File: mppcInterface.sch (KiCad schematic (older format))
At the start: 12 parts, among them J9 Raspberry_Pi_2_3, U1 DAC60508ZRTE, U14 ICE40-LP384-SG32, U2 74HC14, U3 74HC14, U4 INA285

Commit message: Max1932 routed, fpga signal in router. Going to removed Voltage div here
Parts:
- removed D1: S13360-2050VE, s13360-2050ve:S13360-2050VE, symbol s13360-2050ve:S13360-2050VE
- removed R1: 4K99, Resistor_SMD:R_0402_1005Metric, symbol Device:R_US
- removed U2, U3: 74HC14, Package_SO:SOIC-14_3.9x8.7mm_P1.27mm, symbol 74xx:74HC14
- removed U4: INA285, ina28x:TI-DGK-VSSOP-8, symbol ina28x:INA285
- added D1: D, Diode_SMD:D_0402_1005Metric, symbol Device:D
- added TP10: CH5, TestPoint:TestPoint_Bridge_Pitch2.0mm_Drill0.7mm, symbol Connector:TestPoint
- added TP11: CH6, TestPoint:TestPoint_Bridge_Pitch2.0mm_Drill0.7mm, symbol Connector:TestPoint
- added TP12: CH7, TestPoint:TestPoint_Bridge_Pitch2.0mm_Drill0.7mm, symbol Connector:TestPoint
- added TP5: CH0, TestPoint:TestPoint_Bridge_Pitch2.0mm_Drill0.7mm, symbol Connector:TestPoint
- added TP6: CH1, TestPoint:TestPoint_Bridge_Pitch2.0mm_Drill0.7mm, symbol Connector:TestPoint
- added TP7: CH2, TestPoint:TestPoint_Bridge_Pitch2.0mm_Drill0.7mm, symbol Connector:TestPoint
- added TP8: CH3, TestPoint:TestPoint_Bridge_Pitch2.0mm_Drill0.7mm, symbol Connector:TestPoint
- added TP9: CH4, TestPoint:TestPoint_Bridge_Pitch2.0mm_Drill0.7mm, symbol Connector:TestPoint
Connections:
- net labels removed: CH0-A, CH1-A, CH2-A, CH3-A, CH4-A, CH5-A, CH6-A, CH7-A, VBUS
- wire segments 118 -> 123
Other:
- moved on the sheet: U14

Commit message: -5v supply, fpga routed
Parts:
- added C22, C24: 10u, Capacitor_SMD:C_0402_1005Metric, symbol Device:C
- added C23: 1u, Capacitor_SMD:C_0402_1005Metric, symbol Device:C
- added TP2: GND, TestPoint:TestPoint_Bridge_Pitch2.0mm_Drill0.7mm, symbol Connector:TestPoint
- added U2: MIC5504-1.2YM5, Package_TO_SOT_SMD:SOT-23-5, symbol Regulator_Linear:MIC5504-1.2YM5
- added U3: LM2776, Package_TO_SOT_SMD:SOT-23-6, symbol Regulator_SwitchedCapacitor:LM2776
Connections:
- net labels added: -5V
- wire segments 123 -> 147
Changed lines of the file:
@@
 Wire Wire Line
 	6250 4650 6350 4650
+$Comp
+L Regulator_Linear:MIC5504-1.2YM5 U2
+U 1 1 5C3A61F2
+P 1850 6000
+F 0 "U2" H 1850 6367 50  0000 C CNN
+F 1 "MIC5504-1.2YM5" H 1850 6276 50  0000 C CNN
+F 2 "Package_TO_SOT_SMD:SOT-23-5" H 1850 5600 50  0001 C CNN
+F 3 "http://ww1.microchip.com/downloads/en/DeviceDoc/MIC550X.pdf" H 1600 6250 50  0001 C CNN
+	1    1850 6000
+	1    0    0    -1
+$EndComp
+$Comp
+L power:+3V3 #PWR0105
+U 1 1 5C3A62A7
+P 1350 5900
+F 0 "#PWR0105" H 1350 5750 50  0001 C CNN
+F 1 "+3V3" H 1365 6073 50  0000 C CNN
+F 2 "" H 1350 5900 50  0001 C CNN
+F 3 "" H 1350 5900 50  0001 C CNN
+	1    1350 5900
+	1    0    0    -1
+$EndComp
+$Comp
+L power:GND #PWR0106
+U 1 1 5C3A62D4
+P 1850 6350
+F 0 "#PWR0106" H 1850 6100 50  0001 C CNN
+F 1 "GND" H 1855 6177 50  0000 C CNN
+F 2 "" H 1850 6350 50  0001 C CNN
+F 3 "" H 1850 6350 50  0001 C CNN
+	1    1850 6350
+	1    0    0    -1
+$EndComp
+$Comp
+L power:+1V2 #PWR0107
+U 1 1 5C3A6301
+P 2300 5850
+F 0 "#PWR0107" H 2300 5700 50  0001 C CNN
+F 1 "+1V2" H 2315 6023 50  0000 C CNN
+F 2 "" H 2300 5850 50  0001 C CNN
+F 3 "" H 2300 5850 50  0001 C CNN
+	1    2300 5850
+	1    0    0    -1
+$EndComp
+Wire Wire Line
+	1450 6100 1400 6100
+Wire Wire Line
+	1400 6100 1400 5900
+Wire Wire Line
+	1400 5900 1450 5900
+Wire Wire Line
+	2300 5850 2300 5900
+Wire Wire Line
+	2300 5900 2250 5900
+Wire Wire Line
+	1850 6350 1850 6300
+Wire Wire Line
+	1350 5900 1400 5900
+Connection ~ 1400 5900
+$Comp
+L Connector:TestPoint TP?
+U 1 1 5C3D0D7D
+P 10400 5200
+AR Path="/5C210B26/5C3D0D7D" Ref="TP?"  Part="1"
+AR Path="/5C3D0D7D" Ref="TP2"  Part="1"
+F 0 "TP2" H 10458 5320 50  0000 L CNN
+F 1 "GND" H 10458 5229 50  0000 L CNN
+F 2 "TestPoint:TestPoint_Bridge_Pitch2.0mm_Drill0.7mm" H 10600 5200 50  0001 C CNN
+F 3 "~" H 10600 5200 50  0001 C CNN
+	1    10400 5200
+	1    0    0    -1
+$EndComp
+$Comp
+L power:GND #PWR0108
+U 1 1 5C3D0E0F
+P 10400 5250
+F 0 "#PWR0108" H 10400 5000 50  0001 C CNN
+F 1 "GND" H 10405 5077 50  0000 C CNN
+F 2 "" H 10400 5250 50  0001 C CNN
+F 3 "" H 10400 5250 50  0001 C CNN
+	1    10400 5250
+	1    0    0    -1
+$EndComp
+Wire Wire Line
+	10400 5200 10400 5250
+$Comp
+L Regulator_SwitchedCapacitor:LM2776 U3
+U 1 1 5C3D6E4F
+P 2200 4500
+F 0 "U3" H 2350 4300 50  0000 L CNN
+F 1 "LM2776" H 2100 4450 50  0000 L CNN
+F 2 "Package_TO_SOT_SMD:SOT-23-6" H 2250 4150 50  0001 L CNN
+F 3 "http://www.ti.com/lit/ds/symlink/lm2776.pdf" H 350 5750 50  0001 C CNN
+	1    2200 4500
+	1    0    0    -1
+$EndComp
+$Comp
+L power:+5V #PWR0109
+U 1 1 5C3D75DC
+P 2200 4100
+F 0 "#PWR0109" H 2200 3950 50  0001 C CNN
+F 1 "+5V" H 2215 4273 50  0000 C CNN
+F 2 "" H 2200 4100 50  0001 C CNN
+F 3 "" H 2200 4100 50  0001 C CNN
+	1    2200 4100
+	1    0    0    -1
+$EndComp
+$Comp
+L power:GND #PWR0110
+U 1 1 5C3D760D
+P 2200 4950
+F 0 "#PWR0110" H 2200 4700 50  0001 C CNN
+F 1 "GND" H 2205 4777 50  0000 C CNN
+F 2 "" H 2200 4950 50  0001 C CNN
+F 3 "" H 2200 4950 50  0001 C CNN
+	1    2200 4950
+	1    0    0    -1
+$EndComp
+$Comp
+L power:-5V #PWR0111
+U 1 1 5C3D765C
+P 2650 4350
+F 0 "#PWR0111" H 2650 4450 50  0001 C CNN
+F 1 "-5V" H 2665 4523 50  0000 C CNN
+F 2 "" H 2650 4350 50  0001 C CNN
+F 3 "" H 2650 4350 50  0001 C CNN
+	1    2650 4350
+	1    0    0    -1
+$EndComp
+Wire Wire Line
+	1800 4400 1750 4400
+Wire Wire Line
+	1750 4400 1750 4150
+Wire Wire Line
+	1750 4150 2200 4150
+Wire Wire Line
+	2200 4150 2200 4200
+Wire Wire Line
+	2200 4150 2200 4100
+Connection ~ 2200 4150
+Wire Wire Line
+	2600 4400 2650 4400
+Wire Wire Line
+	2650 4400 2650 4350
+Wire Wire Line
+	2200 4900 2200 4950
+$Comp
+L power:GND #PWR0112
+U 1 1 5C3FB554
+P 2650 4950
+F 0 "#PWR0112" H 2650 4700 50  0001 C CNN
+F 1 "GND" H 2655 4777 50  0000 C CNN
+F 2 "" H 2650 4950 50  0001 C CNN
+F 3 "" H 2650 4950 50  0001 C CNN
+	1    2650 4950
+	1    0    0    -1
+$EndComp
+$Comp
+L Device:C C23
+U 1 1 5C3FC376
+P 1650 4650
+AR Path="/5C3FC376" Ref="C23"  Part="1"
+AR Path="/5C210B26/5C3FC376" Ref="C?"  Part="1"
+F 0 "C23" H 1450 4700 50  0000 L CNN
+F 1 "1u" H 1450 4600 50  0000 L CNN
+F 2 "Capacitor_SMD:C_0402_1005Metric" H 1688 4500 50  0001 C CNN
+F 3 "~" H 1650 4650 50  0001 C CNN
+	1    1650 4650
+	1    0    0    -1
+$EndComp
+$Comp
+L Device:C C24
+U 1 1 5C4024E4
+P 2650 4600
+AR Path="/5C4024E4" Ref="C24"  Part="1"
+AR Path="/5C210B26/5C4024E4" Ref="C?"  Part="1"
+F 0 "C24" H 2750 4650 50  0000 L CNN
+F 1 "10u" H 2750 4550 50  0000 L CNN
+F 2 "Capacitor_SMD:C_0402_1005Metric" H 2688 4450 50  0001 C CNN
+F 3 "~" H 2650 4600 50  0001 C CNN
+	1    2650 4600
+	1    0    0    -1
+$EndComp
+$Comp
+L Device:C C22
+U 1 1 5C402572
+P 1300 4650
+AR Path="/5C402572" Ref="C22"  Part="1"
+AR Path="/5C210B26/5C402572" Ref="C?"  Part="1"
+F 0 "C22" H 1100 4700 50  0000 L CNN
+F 1 "10u" H 1050 4600 50  0000 L CNN
+F 2 "Capacitor_SMD:C_0402_1005Metric" H 1338 4500 50  0001 C CNN
+F 3 "~" H 1300 4650 50  0001 C CNN
+	1    1300 4650
+	1    0    0    -1
+$EndComp
+Wire Wire Line
+	1650 4500 1800 4500
+Wire Wire Line
+	1800 4700 1800 4800
+Wire Wire Line
+	1800 4800 1650 4800
+Wire Wire Line
+	2650 4950 2650 4750
+Wire Wire Line
+	2650 4450 2650 4400
+Connection ~ 2650 4400
+$Comp
+L power:GND #PWR0113
+U 1 1 5C41C31D
+P 1300 4900
+F 0 "#PWR0113" H 1300 4650 50  0001 C CNN
+F 1 "GND" H 1305 4727 50  0000 C CNN
+F 2 "" H 1300 4900 50  0001 C CNN
+F 3 "" H 1300 4900 50  0001 C CNN
+	1    1300 4900
+	1    0    0    -1
+$EndComp
+Wire Wire Line
+	1750 4400 1300 4400
+Wire Wire Line
+	1300 4400 1300 4500
+Connection ~ 1750 4400
+Wire Wire Line
+	1300 4800 1300 4900
 Wire Bus Line
 	8750 800  8750 4600

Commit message: Wired up board
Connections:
- net labels added: CLK, GPIO17, GPIO18, GPIO23, GPIO27, RXD, SDA, SDL, TXD
- wire segments 147 -> 169
- no-connect marks 3 -> 8
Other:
- moved on the sheet: TP2

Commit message: Changed inverter IC, added some decoupling
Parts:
- removed C22, C24: 10u, Capacitor_SMD:C_0402_1005Metric, symbol Device:C
- removed C23: 1u, Capacitor_SMD:C_0402_1005Metric, symbol Device:C
- removed D1: D, Diode_SMD:D_0402_1005Metric, symbol Device:D
- removed U3: LM2776, Package_TO_SOT_SMD:SOT-23-6, symbol Regulator_SwitchedCapacitor:LM2776
- added C22, C24: 10u, Capacitor_SMD:C_0402_1005Metric, symbol mppcInterface-rescue:C-Device
- added C23: 1u, Capacitor_SMD:C_0402_1005Metric, symbol mppcInterface-rescue:C-Device
- added C65: 3u3, Capacitor_SMD:C_0402_1005Metric, symbol mppcInterface-rescue:C-Device
- added R1: 1M13, Resistor_SMD:R_0402_1005Metric, symbol Device:R_US
- added R11: 499k, Resistor_SMD:R_0402_1005Metric, symbol Device:R_US
- added U3: LM27761, Package_SON:WSON-8-1EP_2x2mm_P0.5mm_EP0.9x1.6mm, symbol Regulator_SwitchedCapacitor:LM27761
- H1, H2, H3, H4: symbol Mechanical:MountingHole -> mppcInterface-rescue:MountingHole-Mechanical
- J9: symbol Connector:Raspberry_Pi_2_3 -> mppcInterface-rescue:Raspberry_Pi_2_3-Connector
- TP10, TP11, TP12, TP2, TP5, TP6, TP7, TP8, TP9: symbol Connector:TestPoint -> mppcInterface-rescue:TestPoint-Connector
- U2: symbol Regulator_Linear:MIC5504-1.2YM5 -> mppcInterface-rescue:MIC5504-1.2YM5-Regulator_Linear
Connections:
- net labels added: +4V
- net labels removed: -5V
- wire segments 169 -> 180
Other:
- moved on the sheet: TP2, U14

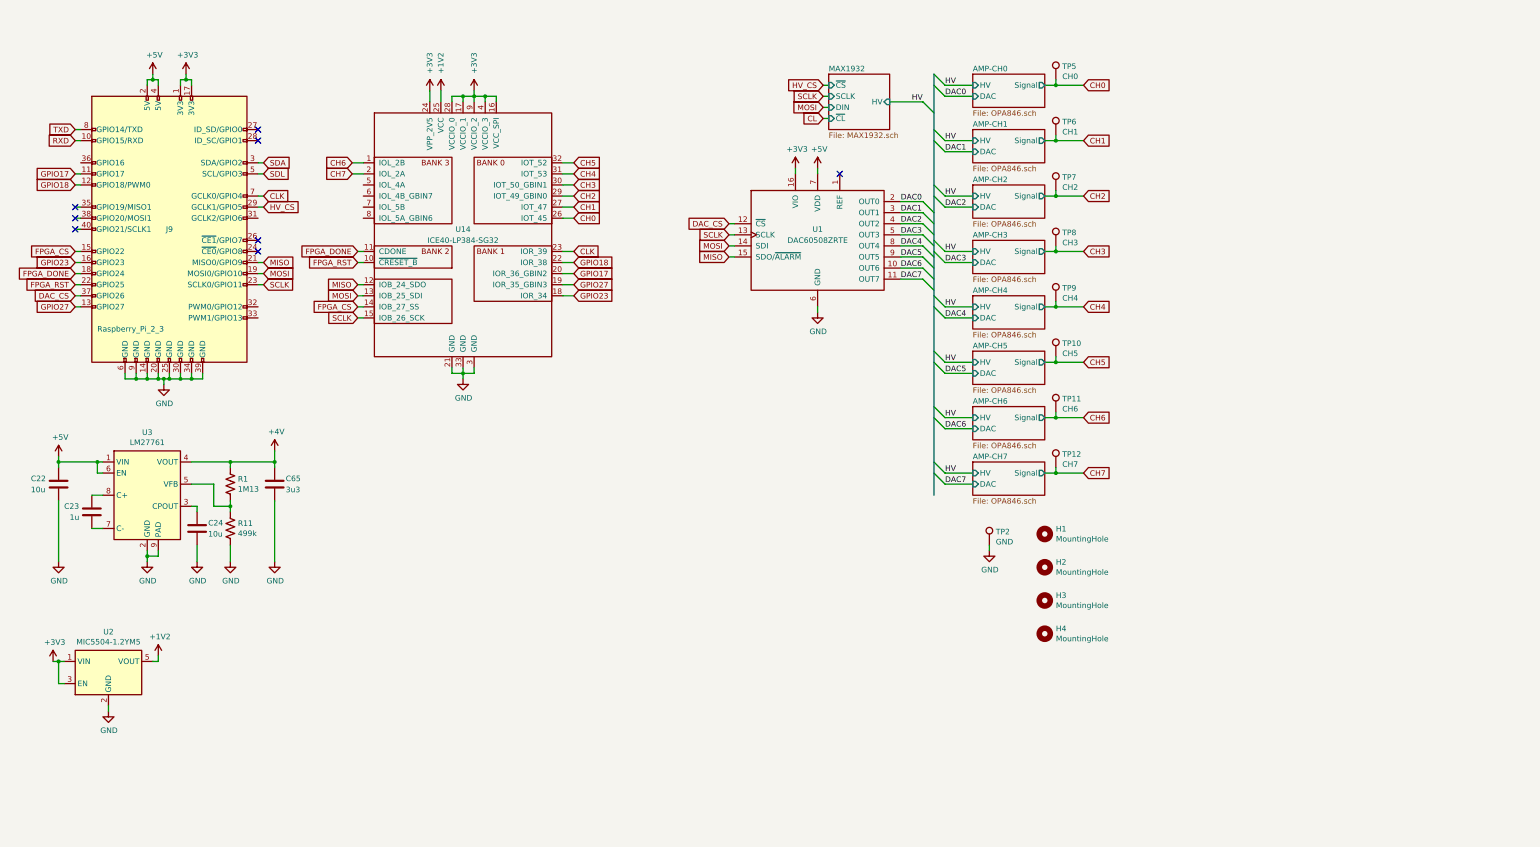
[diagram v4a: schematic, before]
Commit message: Finsihed layout for 1v2
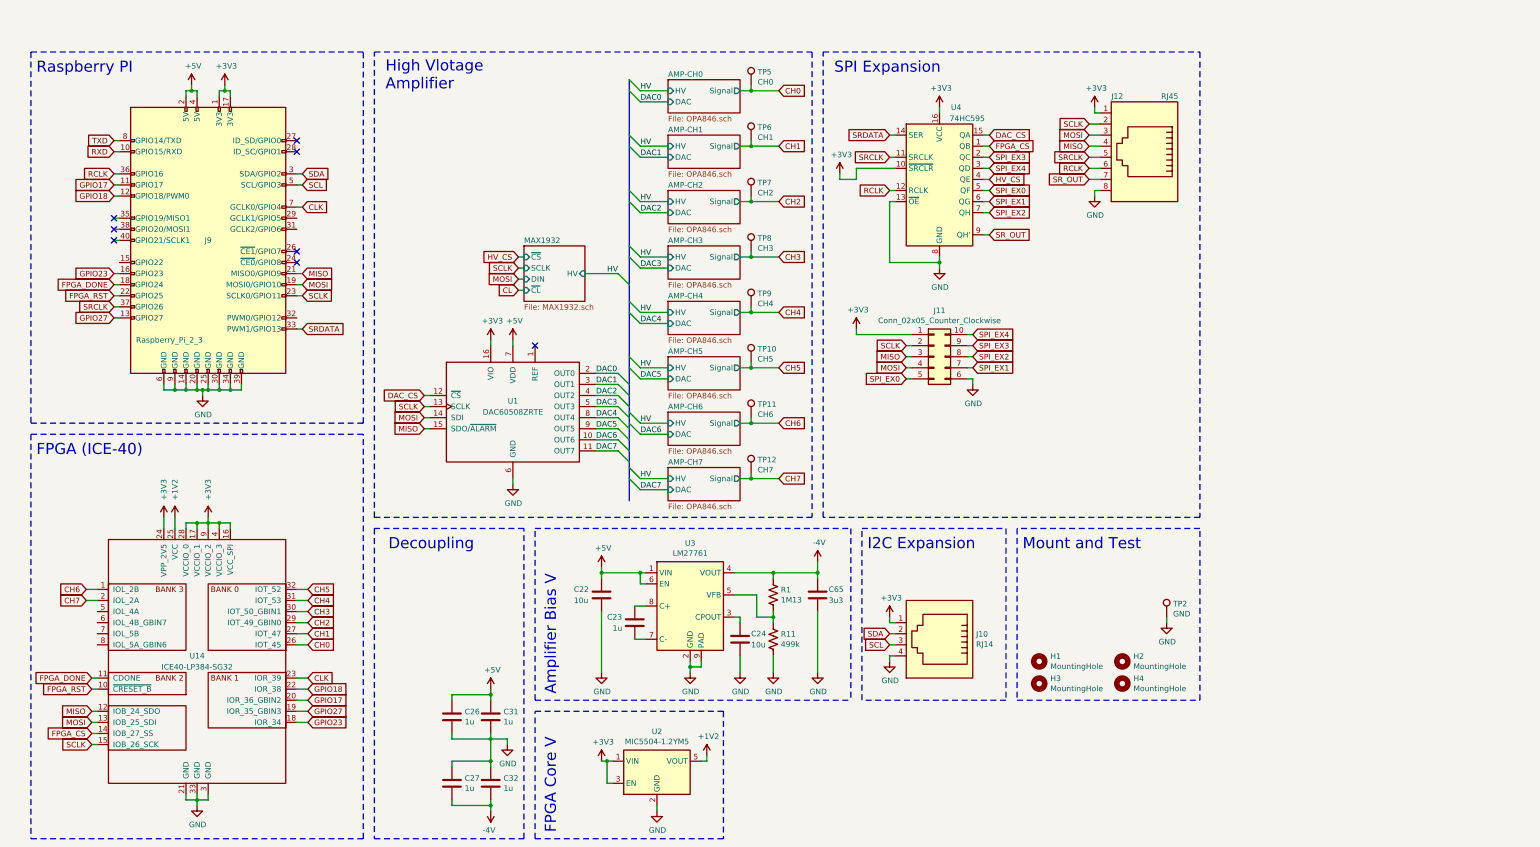
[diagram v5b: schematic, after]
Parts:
- added C26, C27, C31, C32: 1u, Capacitor_SMD:C_0402_1005Metric, symbol Device:C
- added J10: RJ14, Connector_RJ:RJ12_Amphenol_54601, symbol Connector:RJ14
- added J11: Conn_02x05_Counter_Clockwise, Connector_PinHeader_2.54mm:PinHeader_2x05_P2.54mm_Vertical_SMD, symbol Connector_Generic:Conn_02x05_Counter_Clockwise
- added J12: RJ45, Connector_RJ:RJ45_Amphenol_54602-x08_Horizontal, symbol Connector:RJ45
- added U4: 74HC595, Package_SO:TSSOP-16_4.4x5mm_P0.65mm, symbol 74xx:74HC595
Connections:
- net +3V3: now also J10.1, J11.1 (Pin_1), J12.1, U4.10 (~SRCLR), U4.16 (VCC)
- net +5V: now also C26.2, C31.1
- net DAC_CS: now also U4.15 (QA); no longer J9.37 (GPIO26)
- net FPGA_CS: now also U4.1 (QB); no longer J9.15 (GPIO22)
- net GND: now also C26.1, C27.2, C31.2, C32.1, J10.4, J11.6 (Pin_6), J12.8, U4.13 (~OE), U4.8 (GND)
- net HV_CS: now also U4.4 (QE); no longer J9.29 (GCLK1/GPIO5)
- net MISO: now also J11.3 (Pin_3), J12.4
- net MOSI: now also J11.4 (Pin_4), J12.3
- net SCLK: now also J11.2 (Pin_2), J12.2
- net SDA: now also J10.2
- net SRDATA: now reaches J9.33 (PWM1/GPIO13)
- net SRDATA: now also U4.14 (SER)
- net RCLK: now reaches J9.36 (GPIO16)
- net RCLK: now also J12.6, U4.12 (RCLK)
- net +4V renamed -4V
- net -4V: now also C27.1, C32.2
- net SDL renamed SCL
- net SCL: now also J10.3
- new net SPI_EX0: J11.5 (Pin_5), U4.5 (QF)
- new net SPI_EX1: J11.7 (Pin_7), U4.6 (QG)
- new net SPI_EX2: J11.8 (Pin_8), U4.7 (QH)
- new net SPI_EX3: J11.9 (Pin_9), U4.2 (QC)
- new net SPI_EX4: J11.10 (Pin_10), U4.3 (QD)
- new net SRCLK: J12.5, J9.37 (GPIO26), U4.11 (SRCLK)
- new net SR_OUT: J12.7, U4.9 (QH')
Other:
- note added: "Amplifier Bias V"
- note added: "Decoupling"
- note added: "FPGA (ICE-40)"
- note added: "FPGA Core V"
- note added: "High Vlotage\nAmplifier"
- note added: "I2C Expansion"
- note added: "Mount and Test"
- note added: "Raspberry PI"
- note added: "SPI Expansion"
- moved on the sheet: C22, C23, C24, C65, H1, H2, H3, H4, J9, R1, R11, TP10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
